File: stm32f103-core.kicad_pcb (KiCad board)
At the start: 2 copper layers, 30 x 35 mm, 33 parts, among them J1 Conn_01x14, J3 Conn_01x12, J4 Conn_01x12, SW1 SW_Push, U1 STM32F103C8T6, U2 AMS1117-3.3, Y1 O8M, Y2 O32.768K

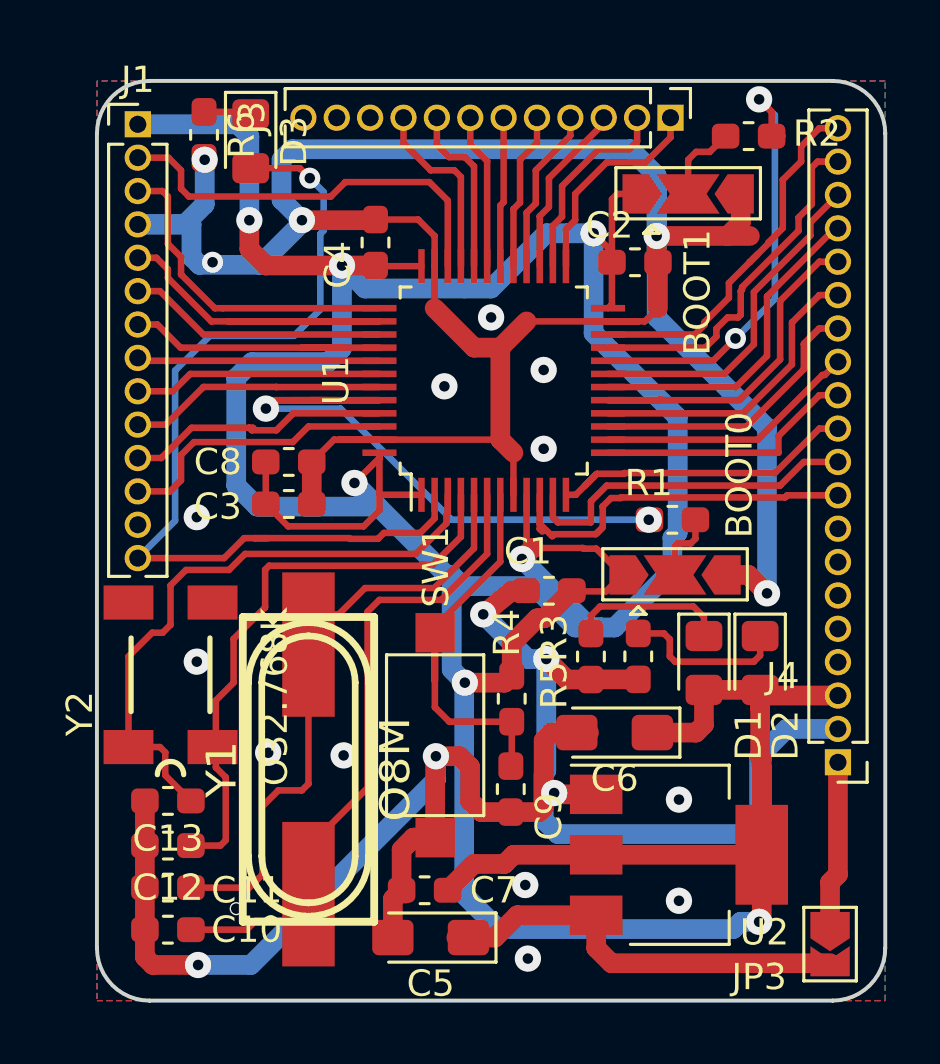
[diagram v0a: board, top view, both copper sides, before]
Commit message: update,
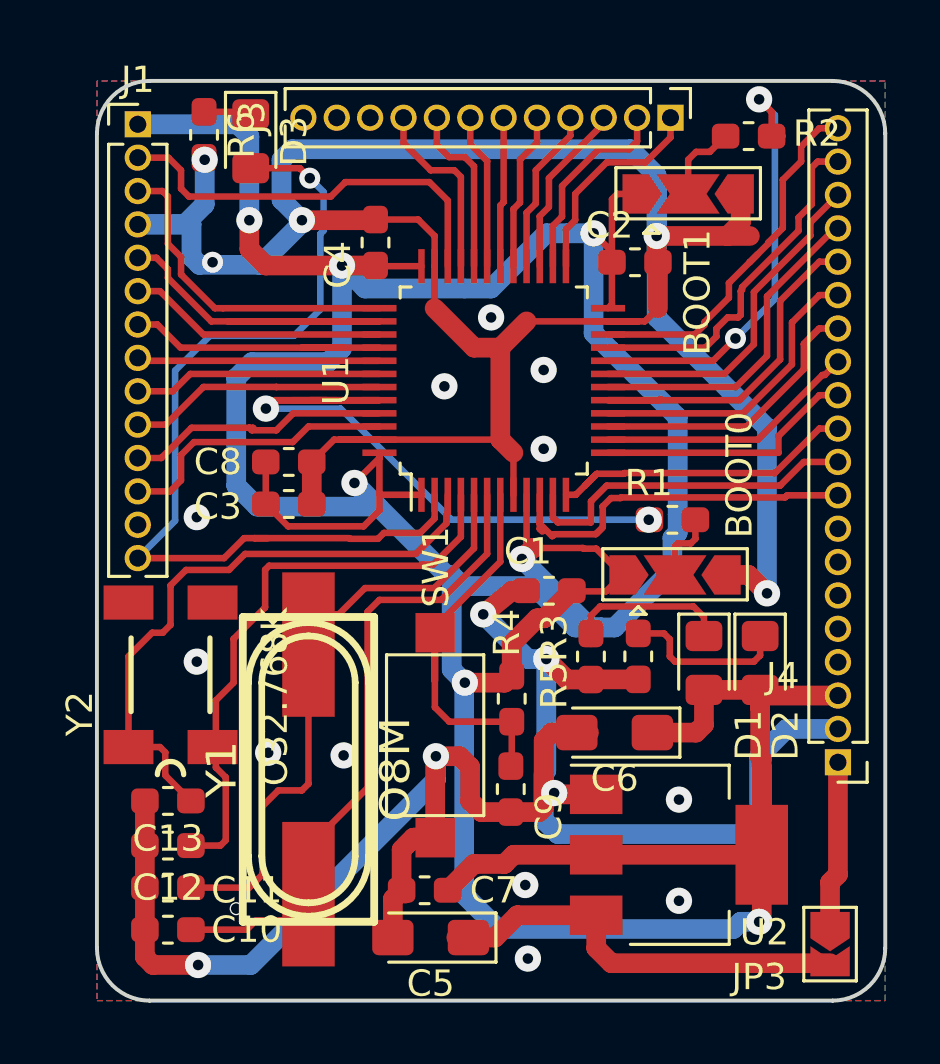
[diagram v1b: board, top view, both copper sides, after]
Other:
- net class 3v3 removed
- net class Default removed
- net class GND removed
- net class PWR removed
